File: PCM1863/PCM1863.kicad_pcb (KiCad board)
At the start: 2 copper layers, 76.2 x 128.5 mm, 70 parts, among them IC1 SN74AUC1G126DCKR, IC2 NCP163ASN330T1G, IC3 NCP163ASN330T1G, IC4 TXB0101DBVT, J1 Conn_01x04_Pin, J11 Conn_01x04_Pin, J2 Conn_01x03_Pin, J3 Conn_01x04_Pin, J4 USB_B_Micro, J5 Conn_01x04_Pin, J6 Conn_01x10_Pin, J7 Conn_01x05_Pin, J8 Conn_02x05_Top_Bottom, U1 PCM1863, Y1 ASE-24.000MHZ-ET, Y2 ASE-22.000MHZ-ET

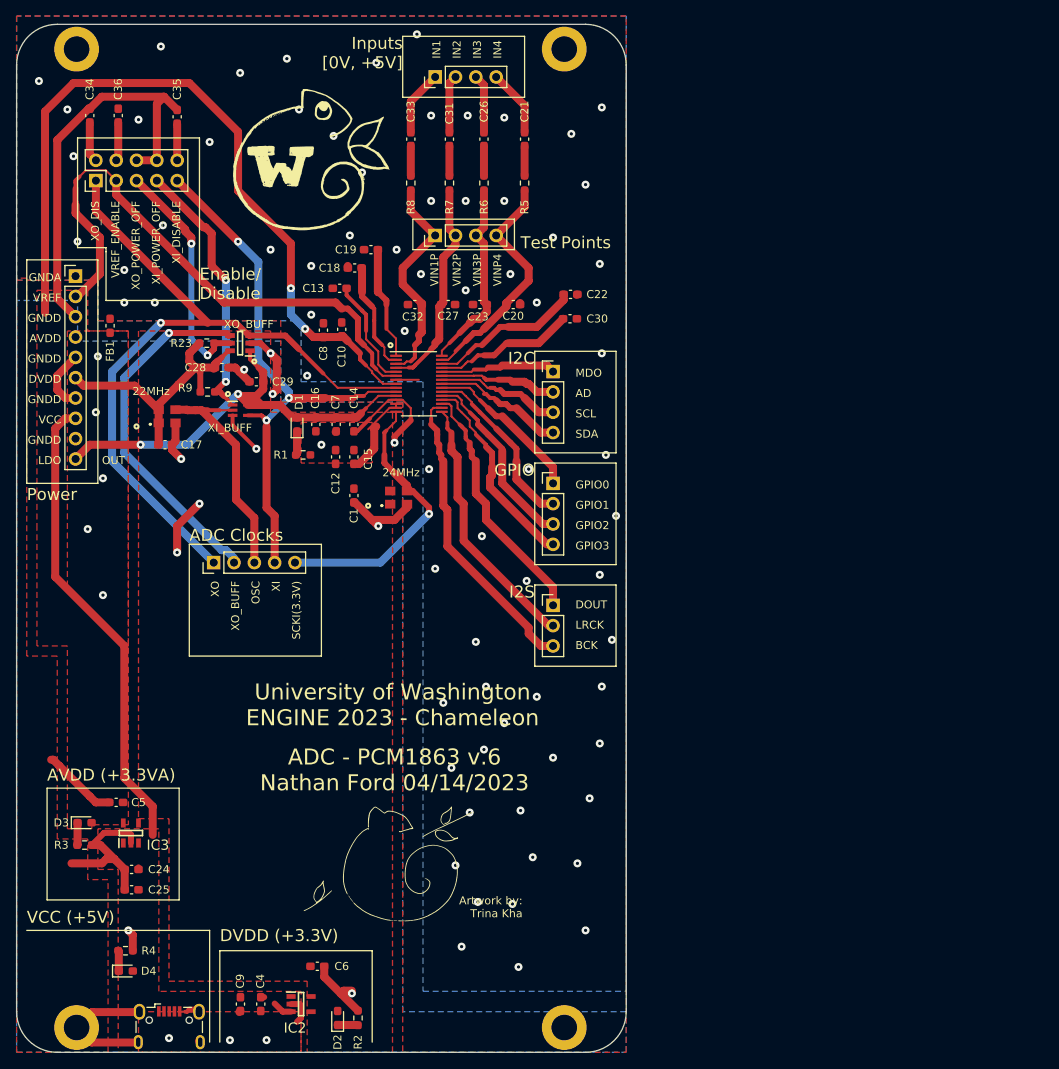
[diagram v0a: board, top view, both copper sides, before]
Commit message: plz work
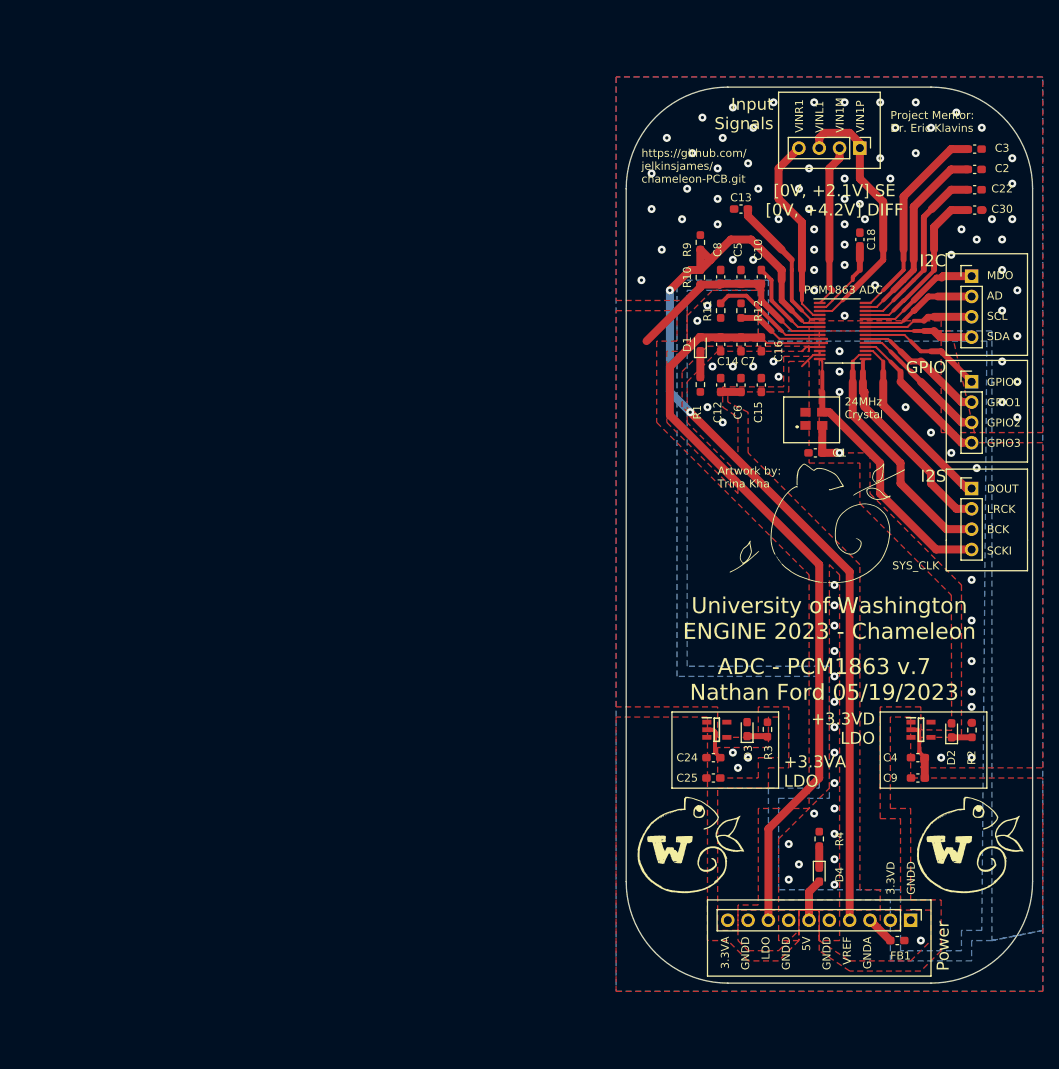
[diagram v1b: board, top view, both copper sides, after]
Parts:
- removed C17: .01uF, Capacitor_SMD:C_0603_1608Metric_Pad1.08x0.95mm_HandSolder
- removed C19: 2.2uF, Capacitor_SMD:C_0603_1608Metric_Pad1.08x0.95mm_HandSolder
- removed C20, C23, C27, C32: 0.01uF, Capacitor_SMD:C_0603_1608Metric_Pad1.08x0.95mm_HandSolder
- removed C21, C26, C31, C33: 10uF, Capacitor_SMD:C_0603_1608Metric_Pad1.08x0.95mm_HandSolder
- removed C28, C29: 0.1uF, Capacitor_SMD:C_0603_1608Metric_Pad1.08x0.95mm_HandSolder
- removed C34, C35: 20pF, Capacitor_SMD:C_0603_1608Metric_Pad1.08x0.95mm_HandSolder
- removed C36: 1uF, Capacitor_SMD:C_0603_1608Metric_Pad1.08x0.95mm_HandSolder
- removed the G*** at (128.5, 39.6)
- removed the G*** at (138.7, 128.5)
- removed H1, H2, H3, H4: MountingHole_Pad, MountingHole:MountingHole_3.2mm_M3_Pad
- removed IC1: SN74AUC1G126DCKR, custom_lib:SOT65P210X110-5N
- removed IC4: TXB0101DBVT, custom_lib:SOT95P280X145-6N
- removed J11, J5: Conn_01x04_Pin, Connector_PinHeader_2.54mm:PinHeader_1x04_P2.54mm_Vertical
- removed J7: Conn_01x05_Pin, Connector_PinHeader_2.54mm:PinHeader_1x05_P2.54mm_Vertical
- removed J8: Conn_02x05_Top_Bottom, Connector_PinHeader_2.54mm:PinHeader_2x05_P2.54mm_Vertical
- removed R23: 4.99k, Resistor_SMD:R_0603_1608Metric_Pad0.98x0.95mm_HandSolder
- removed R5, R6, R7, R8: 100, Resistor_SMD:R_0603_1608Metric_Pad0.98x0.95mm_HandSolder
- removed Y2: ASE-22.000MHZ-ET, custom_lib:ASE24000MHZET
- added C2: 2.2uF, Capacitor_SMD:C_0603_1608Metric_Pad1.08x0.95mm_HandSolder, F.Cu at (211.2, 41.0)
- added C3: 2.2uF, Capacitor_SMD:C_0603_1608Metric_Pad1.08x0.95mm_HandSolder, F.Cu at (211.2, 38.5)
- added G***: LOGO, custom_lib:uw_chameleon, F.Cu at (210.8, 125.3)
- added G***: LOGO, custom_lib:uw_chameleon, F.Cu at (175.9, 125.3)
- added G***: LOGO, custom_lib:blank_chameleon, F.Cu at (192.4, 86.0)
- added R10: 100k, Resistor_SMD:R_0603_1608Metric_Pad0.98x0.95mm_HandSolder, F.Cu at (176.9, 54.5)
- added R11: 100k, Resistor_SMD:R_0603_1608Metric_Pad0.98x0.95mm_HandSolder, F.Cu at (179.5, 58.6)
- added R12: 100k, Resistor_SMD:R_0603_1608Metric_Pad0.98x0.95mm_HandSolder, F.Cu at (182.0, 58.6)
- J2: value Conn_01x03_Pin -> Conn_01x04_Pin; footprint Connector_PinHeader_2.54mm:PinHeader_1x03_P2.54mm_Vertical -> Connector_PinHeader_2.54mm:PinHeader_1x04_P2.54mm_Vertical
- J4: value USB_B_Micro -> Conn_01x04_Pin; footprint Connector_USB:USB_Micro-B_Wuerth_629105150521 -> Connector_PinHeader_2.54mm:PinHeader_1x04_P2.54mm_Vertical
- R9: value 4.99k -> 100k
- moved J6 131.8 mm to (203.2, 134.8), turned to -90 degrees
- moved J4 128.7 mm to (210.8, 67.5)
- moved FB1 124.9 mm to (201.5, 137.4), turned to 180 degrees
- moved C5 102.1 mm to (182.0, 54.4), turned to -90 degrees
- moved C6 89.9 mm to (182.0, 67.9), turned to -90 degrees
- moved C9 89.3 mm to (204.1, 117.1), turned to 0 degrees
- moved R4 87.8 mm to (191.8, 124.7), turned to -90 degrees
- moved C4 87.7 mm to (204.1, 114.5), turned to 0 degrees
- moved D4 87.5 mm to (191.8, 129.1), turned to -90 degrees
- moved R3 86.6 mm to (185.3, 111.0), turned to 90 degrees
- moved R2 84.8 mm to (210.9, 111.1)
- moved D2 84.8 mm to (208.3, 111.1)
- moved IC2 84.7 mm to (204.5, 111.0)
- moved D3 83.6 mm to (182.8, 111.0), turned to 90 degrees
- moved IC3 74.4 mm to (179.0, 111.0), turned to 0 degrees
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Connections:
- J1 pad 2: /VIN2P -> /VIN1M
- J1 pad 3: /VIN3P -> /VIN1P
- J1 pad 4: /VIN4P -> /VINR1
- J4 pad 1: VCC -> /MD4/MISO/GPIO0
- J4 pad 2: unconnected-(J4-D--Pad2) -> /MD5/GPIO1/INTA/DMIN
- J4 pad 3: unconnected-(J4-D+-Pad3) -> /MD6/GPIO2/INTB/DMCLK
- J4 pad 4: unconnected-(J4-ID-Pad4) -> /INT/GPIO3/INTC
- J6 pad 1: GNDA -> GNDD
- J6 pad 10: +1V8 -> +3.3VA
- J6 pad 2: /VREF -> +3V3
- J6 pad 3: GNDD -> GNDA
- J6 pad 4: +3.3VA -> /VREF
- J6 pad 6: +3V3 -> VCC
- J6 pad 8: VCC -> +1V8
- R9 pad 1: +3V3 -> GNDA
- R9 pad 2: /XI_DIS -> /VREF
- U1 pad 1: Net-(U1-VINL2/VIN1M) -> /VIN1M
- U1 pad 29: /VIN4P -> Net-(U1-VINL3/VIN4P)
- U1 pad 30: /VIN3P -> Net-(U1-VINR3/VIN3P)
- U1 pad 4: /VIN2P -> /VINR1
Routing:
- net GNDD: track 149.3 -> 15.4 mm, vias 20 -> 42
- net /XO: track 94.1 -> 14.8 mm, vias 1 -> 0
- net +3.3VA: track 96.2 -> 31.4 mm, vias 2 -> 0
- net /XI: track 71.4 -> 12.8 mm, vias 3 -> 0
- net VCC: track 62.2 -> 5.35 mm
- net /VREF: track 71.8 -> 120.3 mm, vias 0 -> 2
- net /XO_BUFF: track 44.8 -> 0.00 mm, vias 1 -> 0
- net +1V8: track 58.4 -> 101.9 mm, vias 2 -> 0
- net +3V3: track 48.0 -> 6.06 mm
- net /XI_DIS: track 33.7 -> 0.00 mm, vias 2 -> 0
- net /VIN4P: track 29.8 -> 0.00 mm
- net /OSC: track 29.7 -> 0.00 mm
- net /XO_DIS: track 29.4 -> 0.00 mm, vias 2 -> 0
- net /VIN2P: track 26.8 -> 0.00 mm
- net Net-(U1-VINR3/VIN3P): track 0.00 -> 26.1 mm
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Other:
- board size 76.2 x 128.5 mm -> 50.8 x 112 mm
- board text added: "+3.3VA LDO"
- board text added: "+3.3VD LDO"
- board text added: "24MHz Crystal"
- board text added: "3.3VA"
- board text added: "3.3VD"
- board text added: "5V"
- board text added: "ADC - PCM1863 v.7 Nathan Ford 05/19/2023"
- board text added: "Input Signals"
- board text added: "PCM1863 ADC"
- board text added: "Project Mentor: Dr. Eric Klavins"
- board text added: "SCKI"
- board text added: "SYS_CLK"
- board text added: "VIN1M"
- board text added: "VINL1"
- board text added: "VINR1"
- board text added: "[0V, +2.1V] SE [0V, +4.2V] DIFF"
- board text added: "https://github.com/ jelkinsjames/ chameleon-PCB.git"
- board text removed: "22MHz"
- board text removed: "24MHz"
- board text removed: "ADC - PCM1863 v.6 Nathan Ford 04/14/2023"
- board text removed: "ADC Clocks"
- board text removed: "AVDD"
- board text removed: "AVDD (+3.3VA)"
- board text removed: "DVDD"
- board text removed: "DVDD (+3.3V)"
- board text removed: "Enable/ Disable"
- board text removed: "IN1"
- board text removed: "IN2"
- board text removed: "IN3"
- board text removed: "IN4"
- board text removed: "Inputs [0V, +5V]"
- board text removed: "OSC"
- board text removed: "OUT"
- board text removed: "SCKI(3.3V)"
- board text removed: "Test Points"
- board text removed: "VCC"
- board text removed: "VCC (+5V)"
- board text removed: "VIN2P"
- board text removed: "VIN3P"
- board text removed: "VINP4"
- board text removed: "VREF_ENABLE"
- board text removed: "XI"
- board text removed: "XI_BUFF"
- board text removed: "XI_DISABLE"
- board text removed: "XI_POWER_OFF"
- board text removed: "XO"
- board text removed: "XO_BUFF"
- board text removed: "XO_DIS"
- board text removed: "XO_POWER_OFF"
